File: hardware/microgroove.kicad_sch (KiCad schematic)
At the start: 22 parts, among them J1 UJ2-MIBH-4-SMT-TR, J2 SJ1-3513, J3 SJ1-3513, SW1 RotaryEncoder, SW10 SW_Push_Dual, SW11 SW_Push_Dual, SW2 RotaryEncoder, SW3 RotaryEncoder, SW4 RotaryEncoder, SW5 RotaryEncoder, SW6 RotaryEncoder, SW7 SW_Push_Dual, SW8 SW_Push_Dual, SW9 SW_Push_Dual, U1 Pico, U2 H11L1

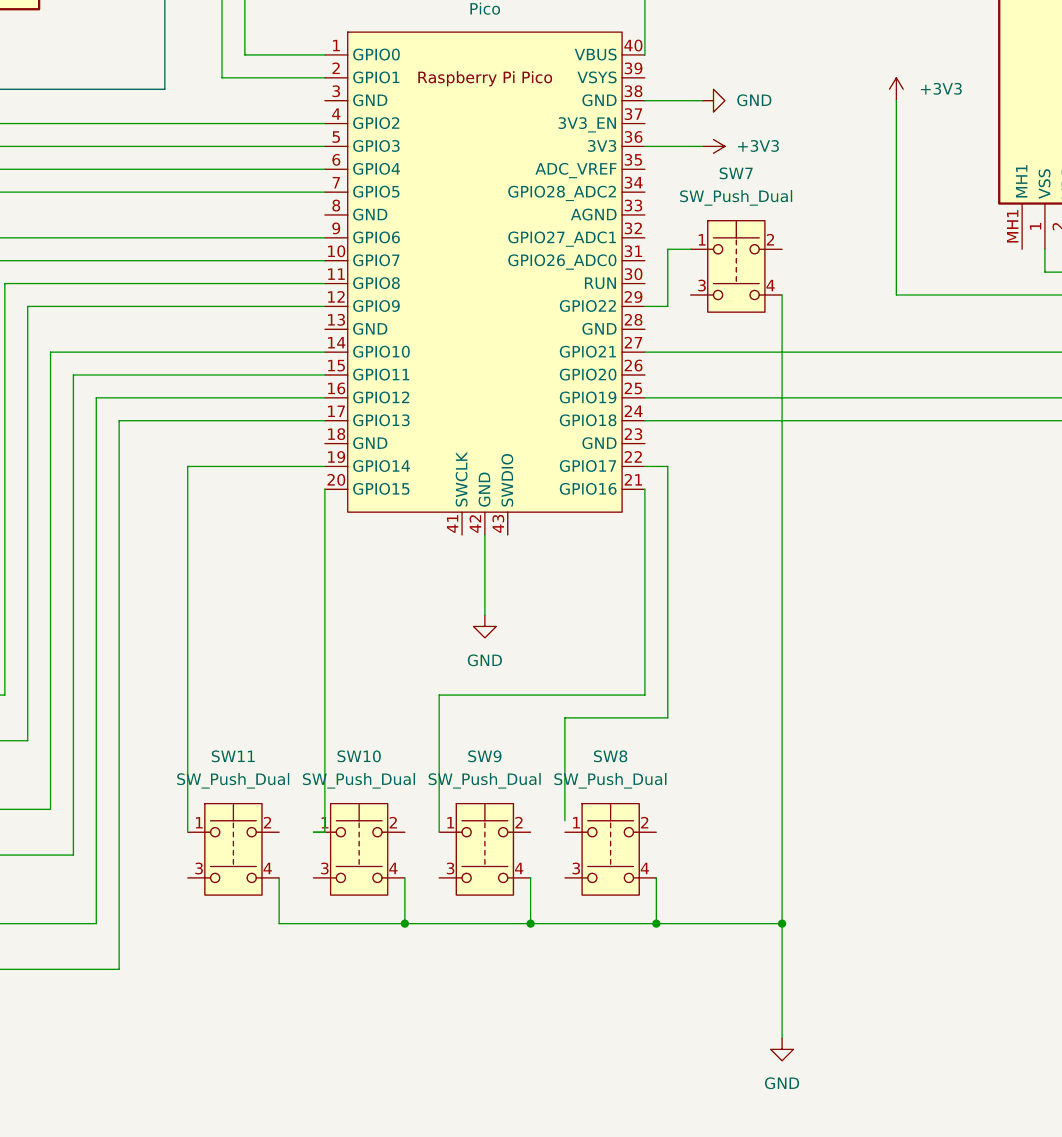
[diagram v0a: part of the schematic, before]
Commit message: Assign footprints for KiCAD schematic symbols
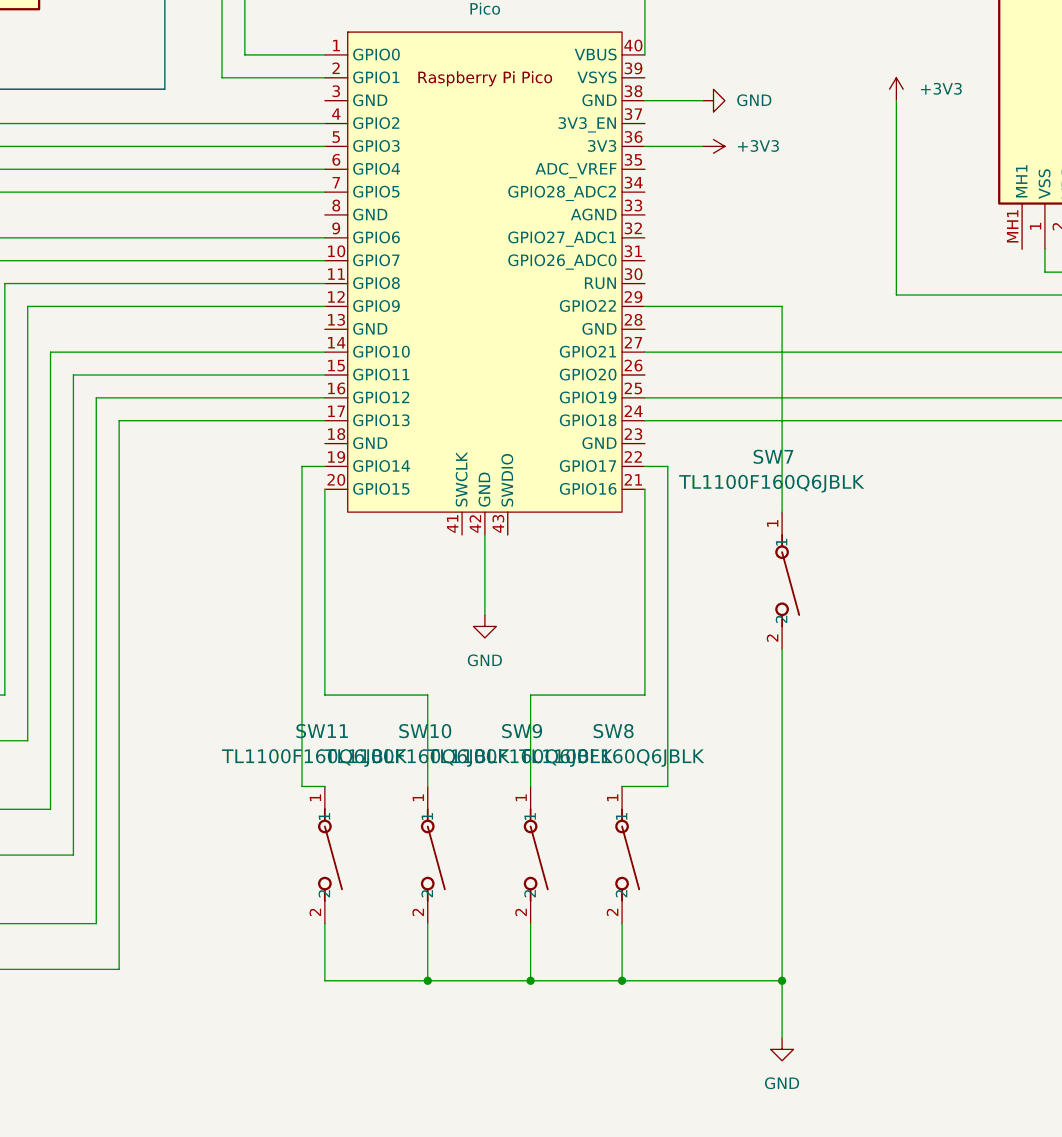
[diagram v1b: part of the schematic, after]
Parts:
- removed SW10, SW11, SW7, SW8, SW9: SW_Push_Dual, symbol Switch:SW_Push_Dual
- added SW10, SW11, SW7, SW8, SW9: TL1100F160Q6JBLK, footprints:SW4_TL1100F160Q6JBLK_EWI, symbol SW4_TL1100F160Q6JBLK_EWI:TL1100F160Q6JBLK
- DS1: footprint NHD2712864WDW3 -> NHD-2.7-12864WDW3:NHD2712864WDW3
- J1: footprint CUIDEVICES_UJ2-MIBH-4-SMT-TR -> UJ2-MIBH-4-SMT-TR:CUIDEVICES_UJ2-MIBH-4-SMT-TR
- J2, J3: footprint SJ1-3513:CUI_SJ1-3513 -> SJ1_3513:CUI_SJ1-3513
- R1, R2, R3, R4: footprint (none) -> Resistor_THT:R_Axial_DIN0207_L6.3mm_D2.5mm_P10.16mm_Horizontal
- SW1, SW2, SW3, SW4, SW5, SW6: footprint (none) -> PEC11R_4215F_S0024:XDCR_PEC11R-4215F-S0024
- U1: footprint RPi_Pico:RPi_Pico_SMD_TH -> MCU_RaspberryPi_and_Boards:RPi_Pico_SMD_TH
- U2: footprint (none) -> Package_DIP:DIP-6_W7.62mm
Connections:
- net GND: now also SW10.2, SW11.2, SW7.2, SW8.2, SW9.2
- net at U1.29 (GPIO22): now also SW7.1
- net at U1.21 (GPIO16): now also SW9.1
- net at U1.19 (GPIO14): now also SW11.1
- net at U1.20 (GPIO15): now also SW10.1
- net at U1.22 (GPIO17): now also SW8.1
